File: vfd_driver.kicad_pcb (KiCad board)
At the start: 2 copper layers, 89.5 x 45.3 mm, 34 parts, among them J1 Input, J2 futaba_7_lt_44z, J3 High Volt, J4 FIL_n, J5 FIL_p, Q3 BC817, Q4 BC807, Q5 BC817, Q6 BC807, U1 74HC595, U2 74HC595, U3 74HC595, U4 74HC595, U5 TBD62783A, U6 TBD62783A, U7 TBD62783A

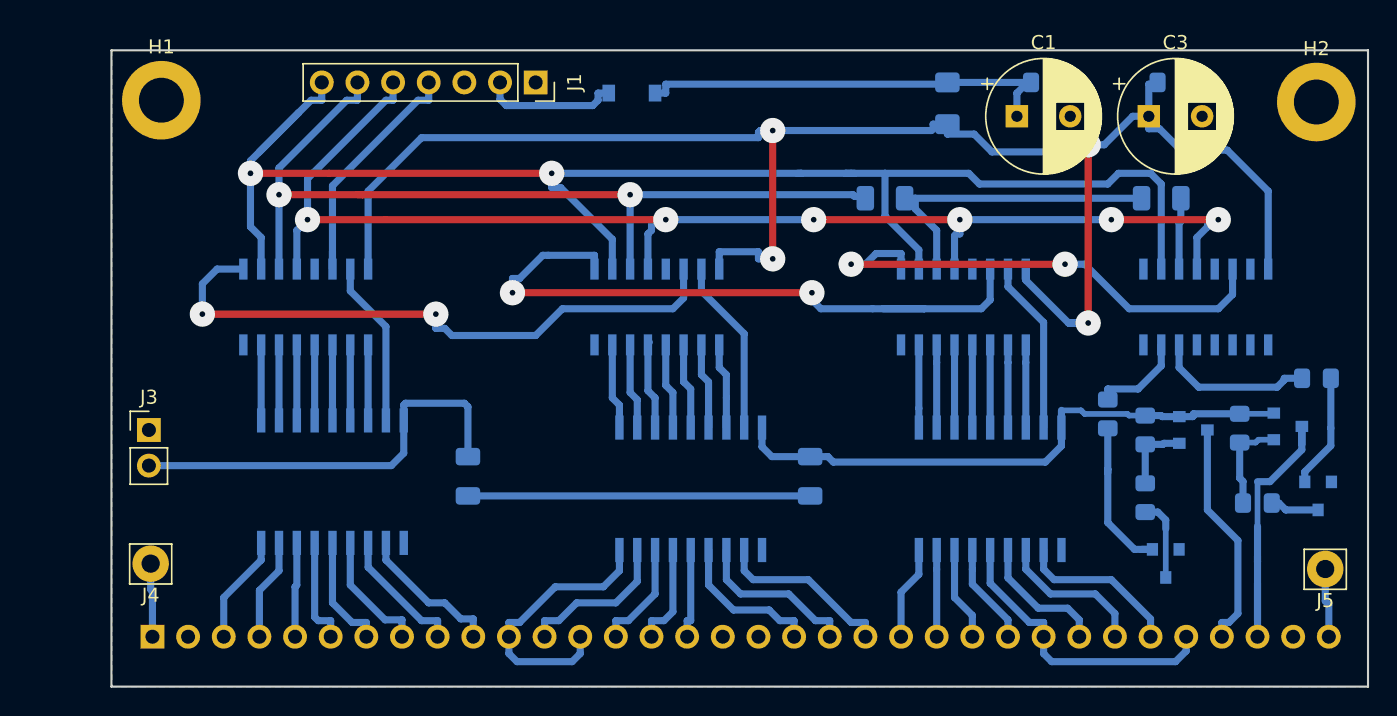
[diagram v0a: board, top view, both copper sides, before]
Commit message: before adding lt1073
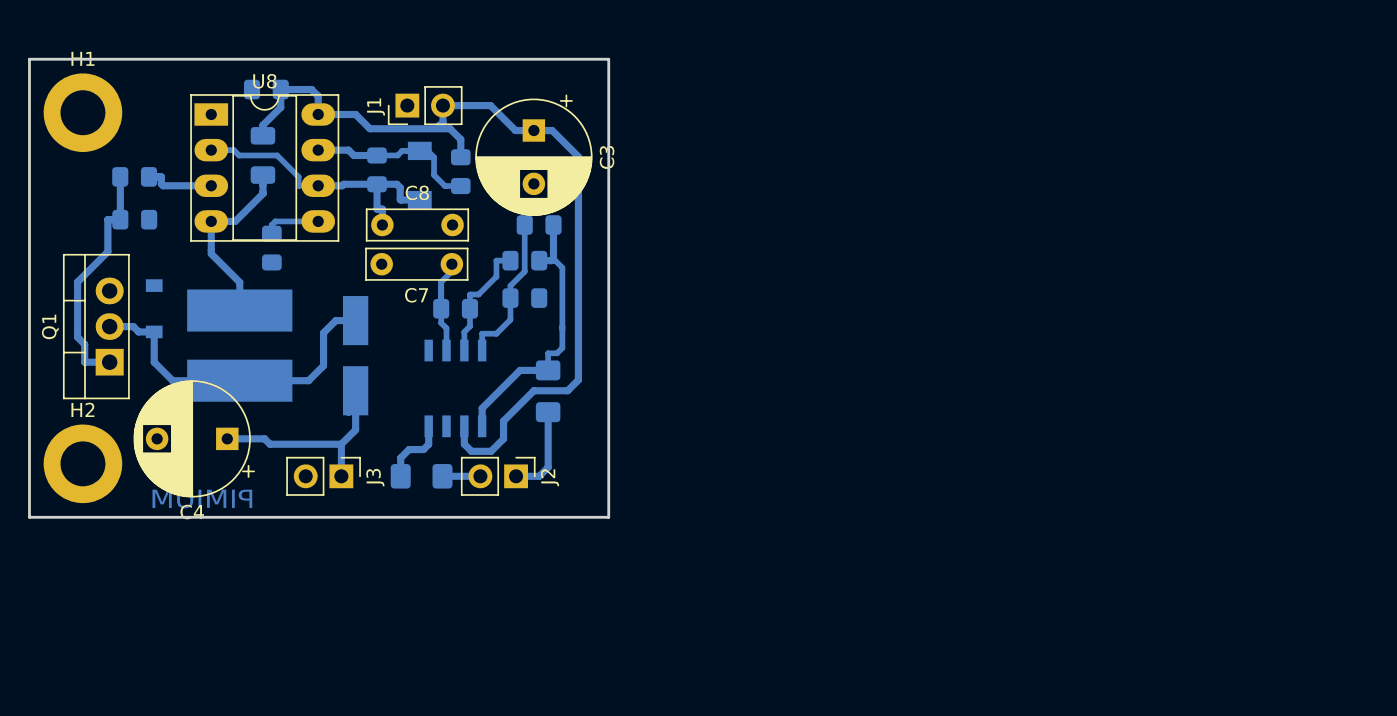
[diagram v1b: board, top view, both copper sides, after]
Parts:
- removed C1: 10u, Capacitor_THT:CP_Radial_D8.0mm_P3.80mm
- removed C2: 100n, Capacitor_SMD:C_0805_2012Metric_Pad1.15x1.40mm_HandSolder
- removed J4: FIL_n, Connector_Pin:Pin_D1.4mm_L8.5mm_W2.8mm_FlatFork
- removed J5: FIL_p, Connector_Pin:Pin_D1.4mm_L8.5mm_W2.8mm_FlatFork
- removed L2: 33, Inductor_SMD:L_1206_3216Metric_Pad1.42x1.75mm_HandSolder
- removed Q3, Q5: BC817, Package_TO_SOT_SMD:SOT-23
- removed Q4, Q6: BC807, Package_TO_SOT_SMD:SOT-23
- removed R10, R7, R8: 33k, Resistor_SMD:R_0805_2012Metric_Pad1.15x1.40mm_HandSolder
- removed R12, R13: 0, Resistor_SMD:R_1206_3216Metric
- removed R6, R9: 100k, Resistor_SMD:R_0805_2012Metric_Pad1.15x1.40mm_HandSolder
- removed U2, U3, U4: 74HC595, Package_SO:SOIC-16_3.9x9.9mm_P1.27mm
- removed U5, U6, U7: TBD62783A, Package_SO:SOP-18_7.0x12.5mm_P1.27mm
- added C4: 10u/63v, Capacitor_THT:CP_Radial_D8.0mm_P5.00mm, F.Cu at (41.9, 56.6)
- added C6: 4n7, Capacitor_SMD:C_0805_2012Metric_Pad1.15x1.40mm_HandSolder, B.Cu at (63.1, 46.6)
- added C7: 1u, Capacitor_THT:C_Rect_L7.0mm_W2.0mm_P5.00mm, F.Cu at (57.9, 44.2)
- added C8: 100n, Capacitor_THT:C_Rect_L7.0mm_W2.0mm_P5.00mm, F.Cu at (53.0, 41.4)
- added C9: 10n, Capacitor_SMD:C_0805_2012Metric_Pad1.15x1.40mm_HandSolder, B.Cu at (45.1, 43.0)
- added D2: SS14, Diode_SMD:D_SMA_Handsoldering, B.Cu at (51.1, 50.7)
- added D3: 1N4148, Diode_SMD:D_MiniMELF, B.Cu at (55.6, 37.9)
- added L1: 330, Choke_SMD:Choke_CD75, B.Cu at (42.8, 50.0)
- added Q1: IRLZ34, Package_TO_SOT_THT:TO-220-3_Vertical, F.Cu at (33.5, 51.2)
- added R14: 0, Resistor_SMD:R_1206_3216Metric, B.Cu at (44.5, 36.4)
- added R15: 22k, Resistor_SMD:R_0805_2012Metric_Pad1.15x1.40mm_HandSolder, B.Cu at (63.1, 43.9)
- added R16: 18, Resistor_SMD:R_1206_3216Metric_Pad1.42x1.75mm_HandSolder, B.Cu at (64.8, 53.2)
- added R17: 18, Resistor_SMD:R_1206_3216Metric_Pad1.42x1.75mm_HandSolder, B.Cu at (55.8, 59.3)
- added R18: 4k7, Resistor_SMD:R_0805_2012Metric_Pad1.15x1.40mm_HandSolder, B.Cu at (52.6, 37.5)
- added R3: 22k, Resistor_SMD:R_0805_2012Metric_Pad1.15x1.40mm_HandSolder, B.Cu at (64.1, 41.4)
- added R4: 10k, Resistor_SMD:R_0805_2012Metric_Pad1.15x1.40mm_HandSolder, B.Cu at (58.2, 47.4)
- added U8: LM555, Package_DIP:DIP-8_W7.62mm_Socket_LongPads, F.Cu at (40.8, 33.5)
- C5: value 10n -> 100n
- D1: value SD103BW -> SD_103BW
- J1: footprint Connector_PinSocket_2.54mm:PinSocket_1x07_P2.54mm_Vertical -> Connector_PinHeader_2.54mm:PinHeader_1x02_P2.54mm_Vertical
- J2: value futaba_7_lt_44z -> FIL; footprint Connector_PinSocket_2.54mm:PinSocket_1x34_P2.54mm_Vertical -> Connector_PinHeader_2.54mm:PinHeader_1x02_P2.54mm_Vertical; moved to F.Cu
- J3: value High Volt -> HV
- R1: value 0 -> 1k; footprint Resistor_SMD:R_1206_3216Metric -> Resistor_SMD:R_0805_2012Metric_Pad1.15x1.40mm_HandSolder
- R2: value 0 -> 100k; footprint Resistor_SMD:R_1206_3216Metric -> Resistor_SMD:R_0805_2012Metric_Pad1.15x1.40mm_HandSolder
- R5: value 33k -> 1k
- U1: value 74HC595 -> LM4871; footprint Package_SO:SOIC-16_3.9x9.9mm_P1.27mm -> Package_SO:SOIC-8_3.9x4.9mm_P1.27mm
- moved H2 91.6 mm to (31.6, 58.4)
- moved R2 73.2 mm to (35.3, 41.0)
- moved C5 64.5 mm to (44.7, 31.8), turned to 180 degrees
- moved R5 62.7 mm to (58.5, 37.6), turned to 270 degrees
- moved U1 53.8 mm to (58.2, 53.0), turned to 270 degrees
- moved R1 53.5 mm to (35.3, 38.0)
- moved C3 43.8 mm to (63.8, 34.7), turned to 270 degrees
- moved D1 37.3 mm to (36.7, 47.4), turned to 90 degrees
- moved J2 28.3 mm to (62.5, 59.3)
- moved J3 14.1 mm to (50.0, 59.3), turned to 270 degrees
- moved J1 9.29 mm to (54.7, 32.9), turned to 90 degrees
- moved H1 5.66 mm to (31.6, 33.4)
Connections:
- C3 pad 1: VCC -> +5V
- C5 pad 1: VCC -> +5V
- D1 pad 2: VDD -> GND
- J1 pad 2: VDD -> +5V
- J2 pad 1: Net-(J2-Pad1) -> /FIL_n
- J2 pad 2: (no net) -> /FIL_p
- J3 pad 1: GND -> +36V
- J3 pad 2: +36V -> GND
- R1 pad 1: /SRCLK -> Net-(Q1-Pad1)
- R1 pad 2: /SRCLK -> /HV
- R2 pad 1: /SRCLK -> Net-(Q1-Pad1)
- R2 pad 2: /SRCLK -> GND
- R5 pad 1: /Q4G -> +5V
- U1 pad 1: (no net) -> GND
- U1 pad 2: (no net) -> Net-(C7-Pad1)
- U1 pad 3: (no net) -> Net-(R15-Pad2)
- U1 pad 4: (no net) -> Net-(C6-Pad1)
- U1 pad 5: (no net) -> Net-(R15-Pad1)
- U1 pad 6: /Q4G -> +5V
- U1 pad 7: /Q4H -> GND
- U1 pad 8: GND -> Net-(R17-Pad1)
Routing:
- net VCC: track 119.9 -> 0.00 mm, vias 4 -> 0
- net /~SRCLR: track 109.7 -> 0.00 mm, vias 2 -> 0
- net /RCLK: track 94.4 -> 0.00 mm, vias 6 -> 0
- net /SRCLK: track 93.5 -> 0.00 mm, vias 2 -> 0
- net +5V: track 0.00 -> 81.7 mm
- net +36V: track 95.8 -> 18.2 mm
- net /Q1: track 48.7 -> 0.00 mm, vias 2 -> 0
- net /Q0: track 45.6 -> 0.00 mm, vias 2 -> 0
- net /Q2: track 35.3 -> 0.00 mm, vias 2 -> 0
- net Net-(R15-Pad1): track 0.00 -> 27.1 mm
- net /G1: track 21.3 -> 0.00 mm
- net Net-(C8-Pad1): track 0.00 -> 21.2 mm
- net /S10: track 21.1 -> 0.00 mm
- net /G5: track 19.9 -> 0.00 mm
- net Net-(Q1-Pad1): track 0.00 -> 17.9 mm
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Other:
- board size 89.5 x 45.3 mm -> 41.3 x 32.6 mm
- board text removed: "VFD-DRIVER"
